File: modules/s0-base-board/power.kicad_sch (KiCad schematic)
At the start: 25 parts, among them J2 Screw_Terminal_01x02, J3 BAT_JST_01x02, Q1 PMOS, U1 MCP73831-2-OT, U2 XL1509-5.0, U3 LM2575S-3.3(UMW)

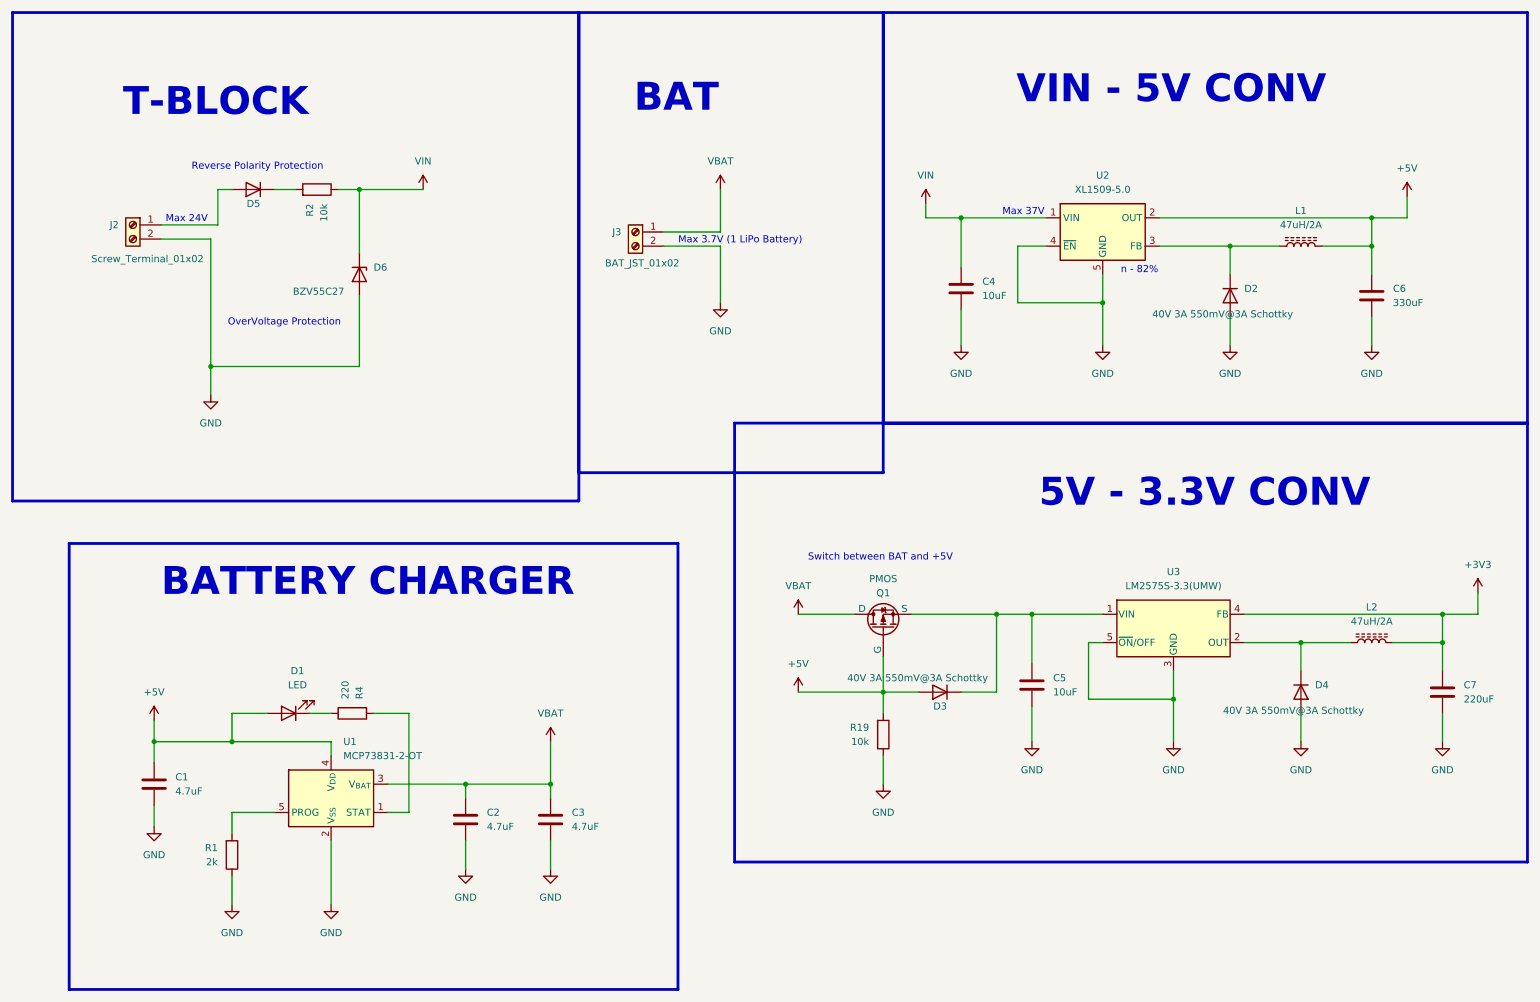
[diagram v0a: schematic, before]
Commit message: Reviewed Changes made
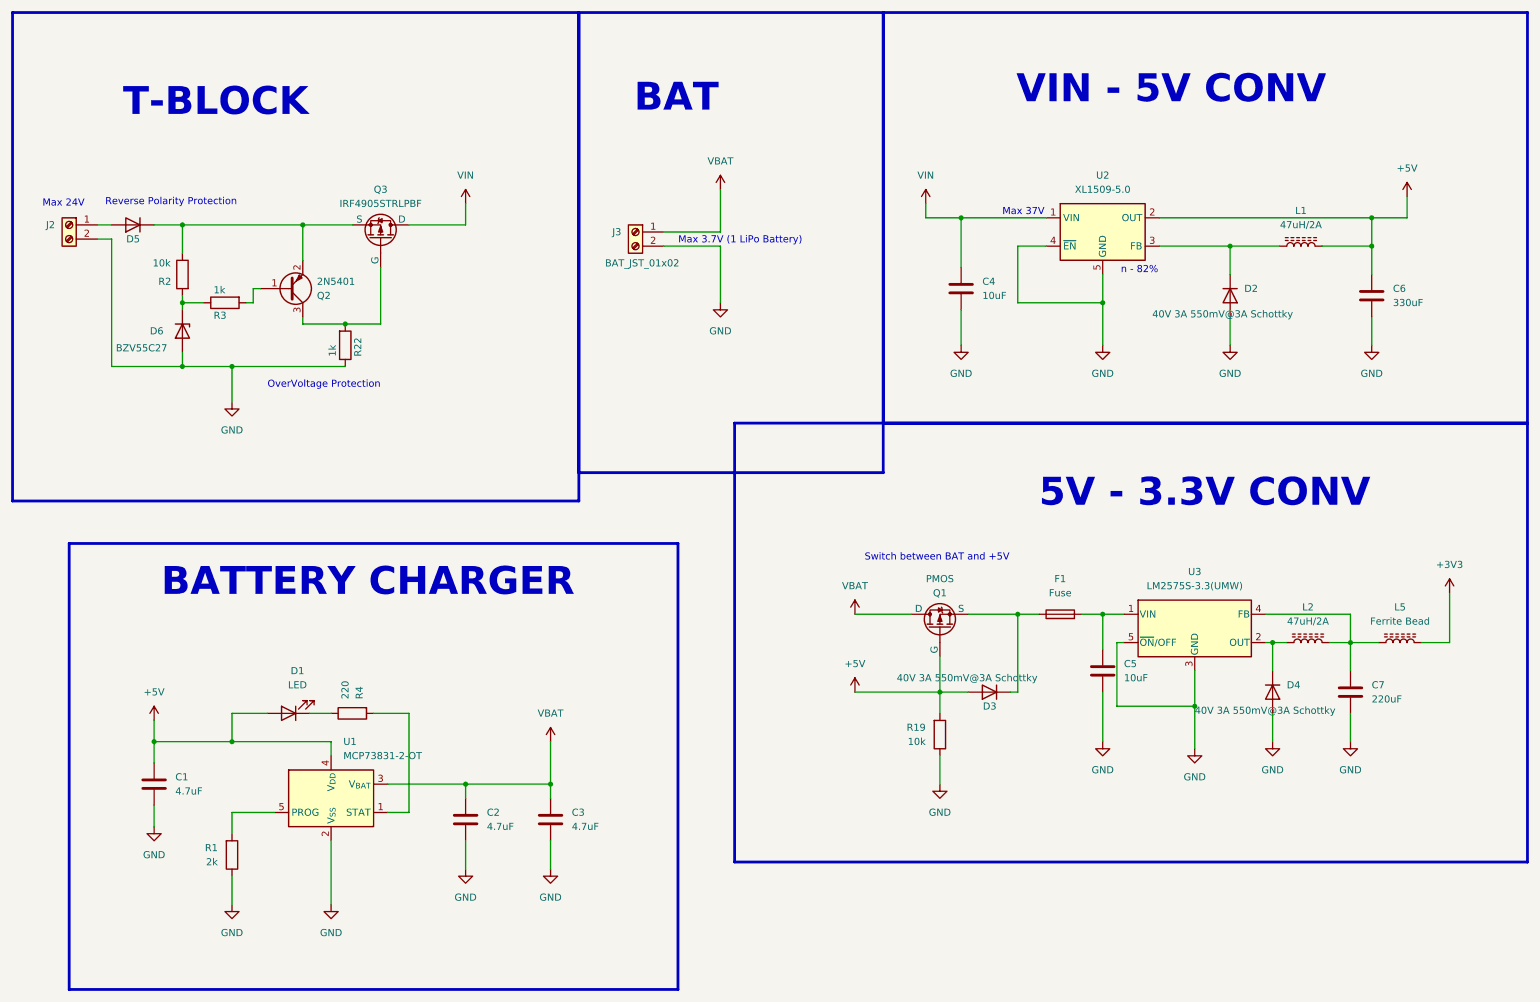
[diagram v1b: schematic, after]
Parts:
- added F1: Fuse, Module:FUSC3115X66N, symbol Device:Fuse
- added L5: Ferrite Bead, Module:BEADC3216X130N, symbol Device:L_Ferrite
- added Q2: 2N5401, Module:SOT95P230X117-3N, symbol BeagleBone Capes:2N5401
- added Q3: IRF4905STRLPBF, Module:TRANS_IRF3205S, symbol Simulation_SPICE:PMOS
- added R22, R3: 1k, Resistor_SMD:R_0402_1005Metric, symbol Device:R
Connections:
- net +3V3: now also L5.2; no longer C7.1, L2.2, U3.4 (FB)
- net GND: now also R22.1
- net VIN: now also Q3.1 (D); no longer D6.1 (K), R2.1
- net at C5.1, U3.1 (VIN): now also F1.2; no longer D3.1 (K), Q1.3 (S)
- net at R2.2: now also D6.1 (K), R3.1; no longer D5.1 (K)
- new net: Q2.3 (C), Q3.2 (G), R22.2
- new net: C7.1, L2.2, L5.1, U3.4 (FB)
- new net: D3.1 (K), F1.1, Q1.3 (S)
- new net: D5.1 (K), Q2.2 (E), Q3.3 (S), R2.1
- new net: Q2.1 (B), R3.2
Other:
- moved on the sheet: C5, C7, D3, D4, D5, D6, J2, L2, Q1, R19, R2, U3
